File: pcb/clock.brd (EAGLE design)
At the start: 76.2 x 71.1 mm, 17 parts, among them IC1 74AHCT125, U1 ESP-01, U2 LD1117V33

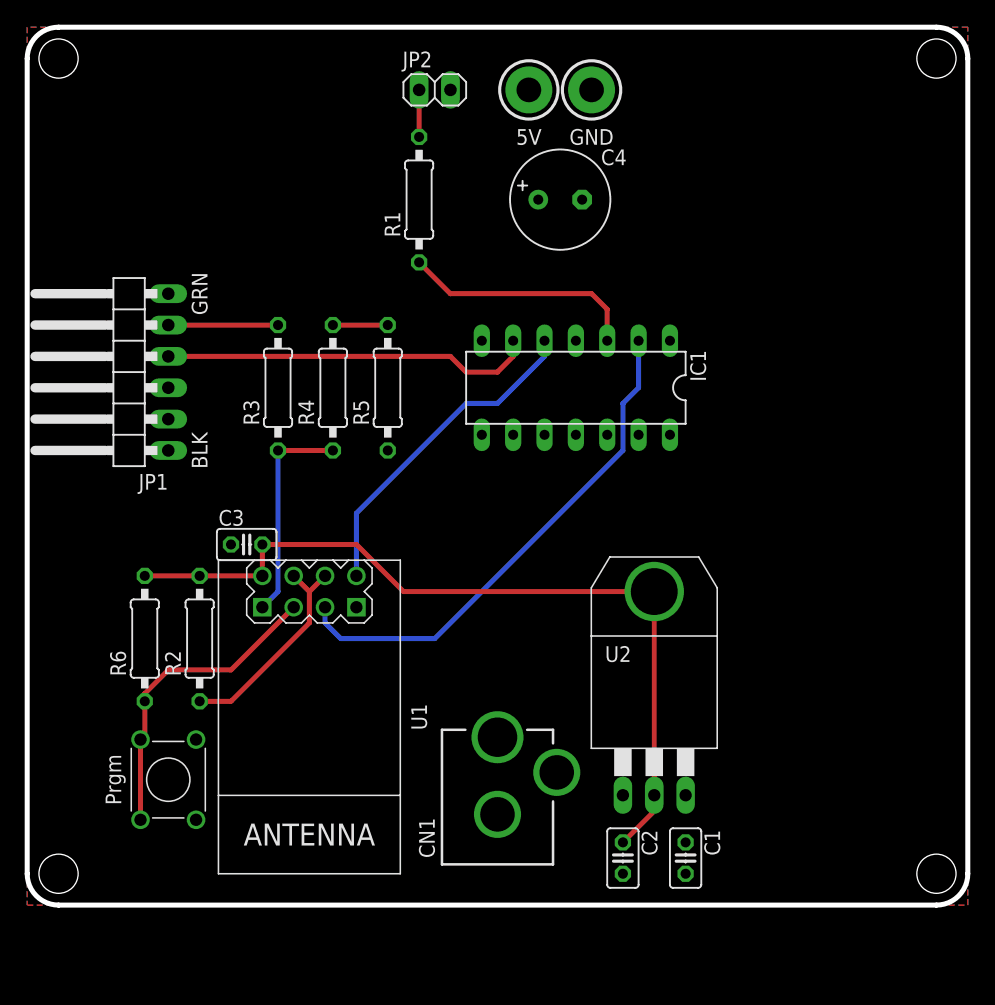
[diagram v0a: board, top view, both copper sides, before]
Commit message: Linearized the board layout
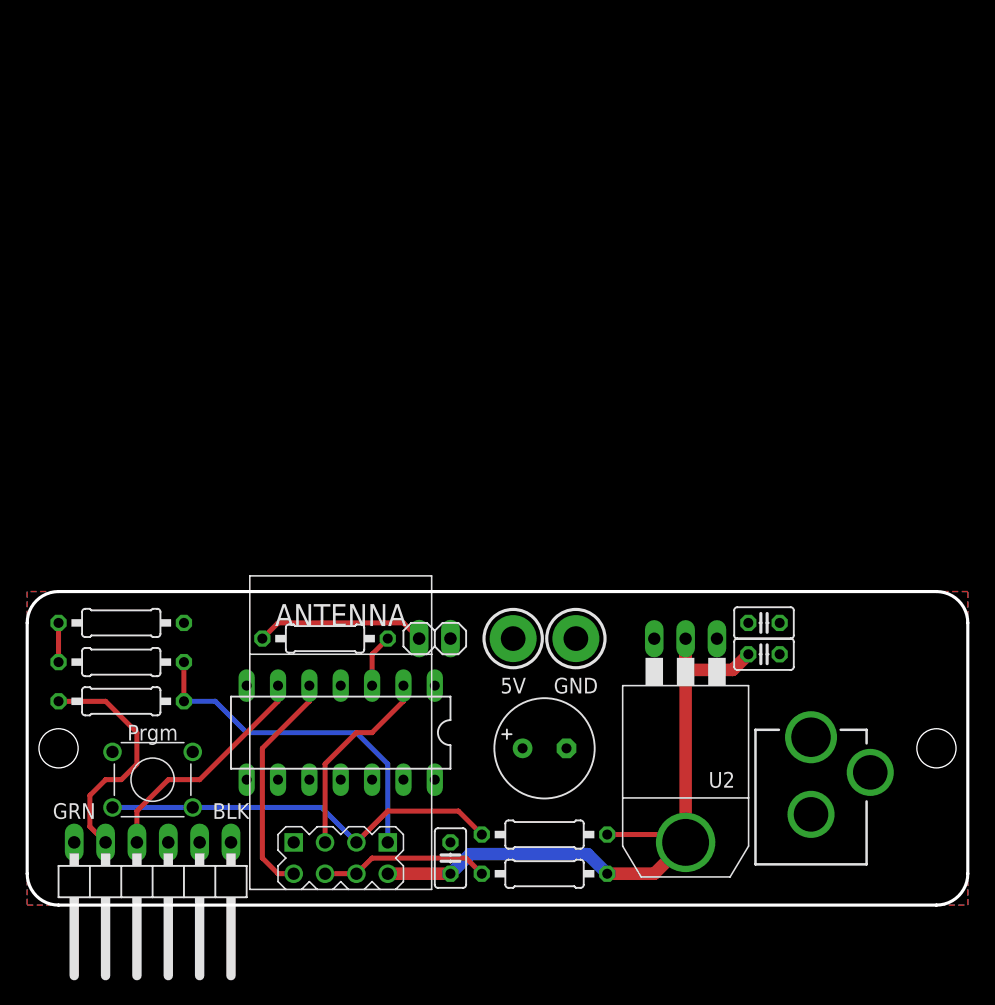
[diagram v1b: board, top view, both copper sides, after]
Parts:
- moved C4 44.5 mm to (41.9, 12.7)
- moved JP2 44.5 mm to (33.0, 21.6)
- moved JP1 42.0 mm to (10.2, 1.27), turned to 180 degrees
- moved R1 36.4 mm to (24.1, 21.6), turned to 180 degrees
- moved R6 36.1 mm to (41.9, 5.71), turned to 0 degrees
- moved IC1 33.8 mm to (25.4, 14.0)
- moved R2 33.8 mm to (41.9, 2.54), turned to 0 degrees
- moved C3 30.3 mm to (34.3, 3.81), turned to 90 degrees
- moved R5 28.8 mm to (7.62, 22.9), turned to 180 degrees
- moved R3 28.4 mm to (7.62, 16.5), turned to 180 degrees
- moved R4 28.1 mm to (7.62, 19.7), turned to 0 degrees
- moved CN1 25.4 mm to (63.5, 0.00)
- moved C2 20.1 mm to (59.7, 20.3), turned to 0 degrees
- moved C1 20.1 mm to (59.7, 22.9), turned to 180 degrees
- moved U2 5.68 mm to (53.3, 17.8), turned to 180 degrees
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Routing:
- net GPIO2: track 41.7 -> 16.1 mm
- net NP_DATA: track 19.4 -> 4.34 mm
- net TXD_5V: track 30.3 -> 18.9 mm
- net RXD_3V3: track 17.7 -> 28.1 mm
- net RXD_5V: track 8.89 -> 19.1 mm
- net N$1: track 3.81 -> 13.8 mm
- net VCC: track 66.8 -> 57.7 mm
- net TXD_3V3: track 26.9 -> 18.6 mm
- net GPIO0: track 25.3 -> 32.9 mm
- net N$2: track 17.7 -> 13.8 mm
- net N$3: track 4.45 -> 3.18 mm
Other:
- board size 76.2 x 71.1 mm -> 76.2 x 25.4 mm
